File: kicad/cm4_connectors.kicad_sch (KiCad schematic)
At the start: 8 parts, among them CN15 KF2EDGR-2.54-10P, J3 Header-Male-2.54_2x3, U14 2541WV-2X12P, U15 74LVC1G07SE-7, U16 74LVC1G07SE-7

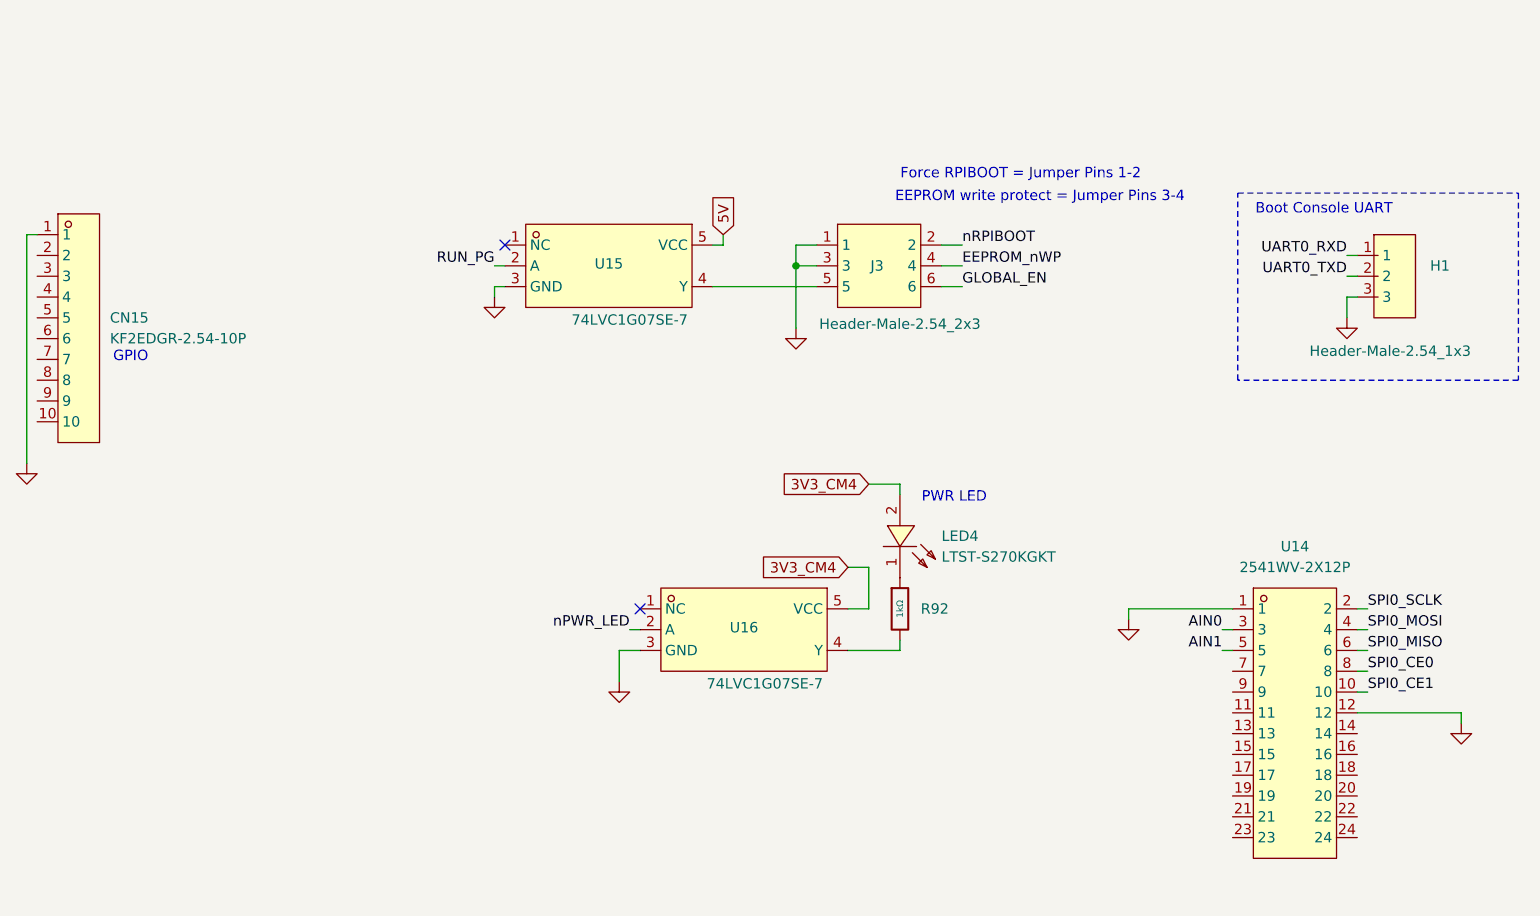
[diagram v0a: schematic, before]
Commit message: CM4 schematic changes, before renumbering
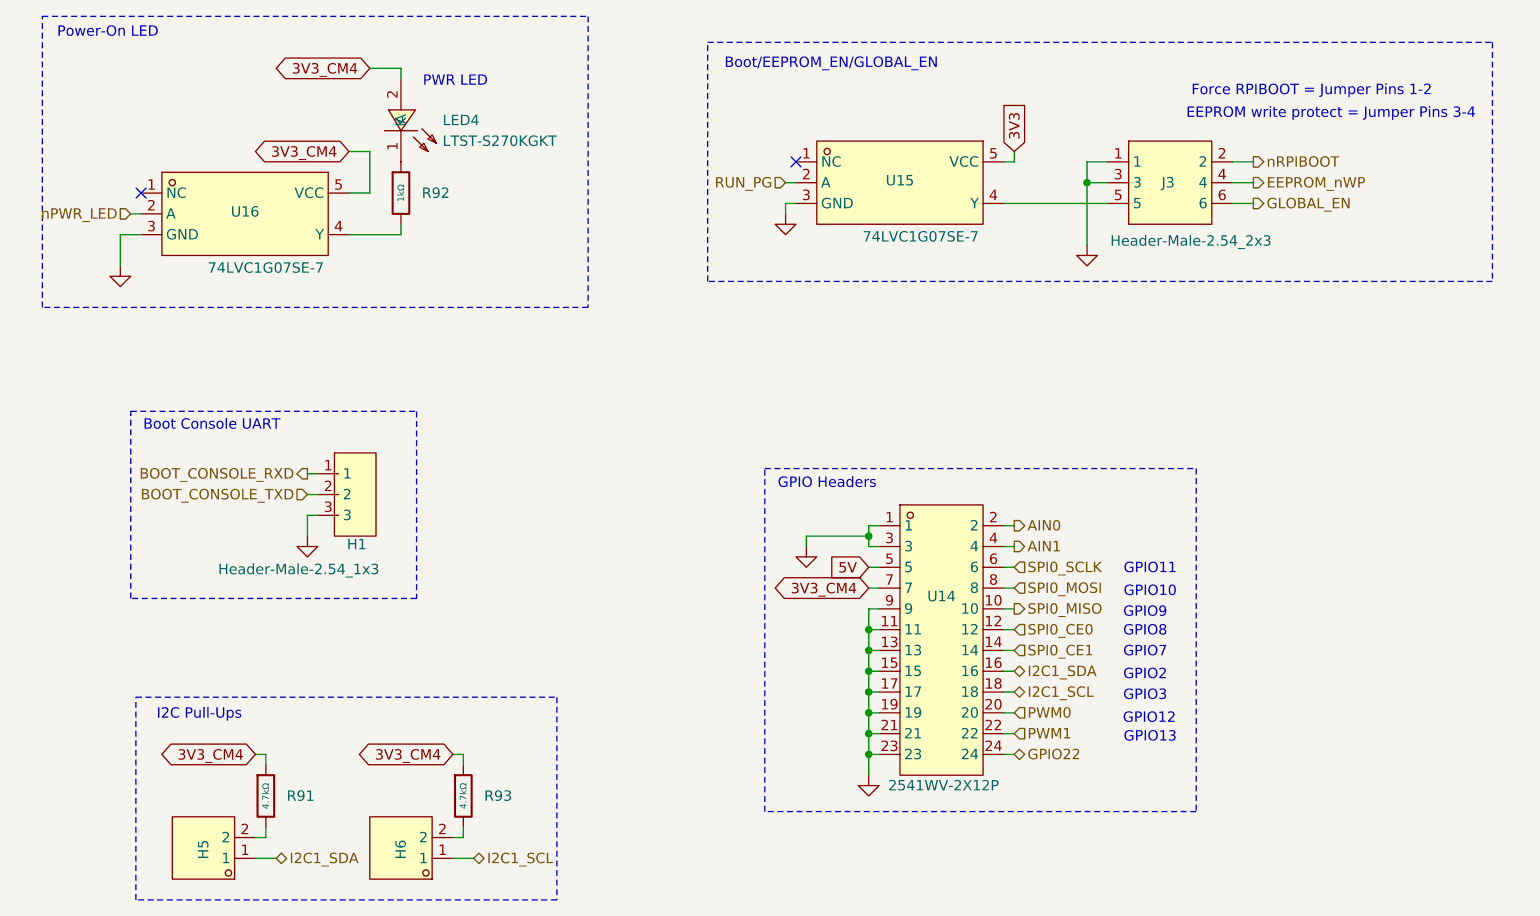
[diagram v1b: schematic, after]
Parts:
- removed CN15: KF2EDGR-2.54-10P, MyParts:CONN-TH_10P-P2.54_KF2EDGR-2.54-10P, symbol MyParts:KF2EDGR-2.54-10P
- added H5, H6: 210S-1*2P L=11.6MMGold-plated black, MyParts:HDR-TH_2P-P2.54-V-M-1, symbol MyParts:210S-1*2PL=11.6MMGold-platedblack
- added R91, R93: 4.7kΩ, PCM_JLCPCB:R_0402, symbol PCM_JLCPCB-Resistors:0402,4.7kΩ
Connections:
- net 3V3_CM4: now also U14.7, R91.1, R93.1
- net 5V: now also U14.5; no longer U15.5 (VCC)
- net AIN0: now also U14.2; no longer U14.3
- net AIN1: now also U14.4; no longer U14.5
- net GND: now also U14.11, U14.13, U14.15, U14.17, U14.19, U14.21, U14.23, U14.3, U14.9; no longer U14.12
- net SPI0_CE0: now also U14.12; no longer U14.8
- net SPI0_CE1: now also U14.14; no longer U14.10
- net SPI0_MISO: now also U14.10; no longer U14.6
- net SPI0_MOSI: now also U14.8; no longer U14.4
- net SPI0_SCLK: now also U14.6; no longer U14.2
- net I2C1_SDA: now reaches U14.16
- net I2C1_SDA: now also H5.1
- net I2C1_SCL: now reaches U14.18
- net I2C1_SCL: now also H6.1
- net PWM0: now reaches U14.20
- net PWM1: now reaches U14.22
- net GPIO22: now reaches U14.24
- net UART0_RXD renamed BOOT_CONSOLE_RXD
- net UART0_TXD renamed BOOT_CONSOLE_TXD
- new net: H6.2, R93.2
- new net: H5.2, R91.2
- new net 3V3: U15.5 (VCC)
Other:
- note added: "Boot/EEPROM_EN/GLOBAL_EN"
- note added: "GPIO Headers"
- note added: "GPIO10"
- note added: "GPIO11"
- note added: "GPIO12"
- note added: "GPIO13"
- note added: "GPIO2"
- note added: "GPIO3"
- note added: "GPIO7"
- note added: "GPIO8"
- note added: "GPIO9"
- note added: "I2C Pull-Ups"
- note added: "Power-On LED"
- note removed: "GPIO"
- moved on the sheet: H1, J3, R92, U14, U15, U16
